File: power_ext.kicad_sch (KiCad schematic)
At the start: 11 parts, among them J1 Conn_01x01, J2 Conn_01x01, J3 Conn_01x01, J4 Conn_01x01, J5 Conn_01x01, J6 Conn_01x01, U132 TLV9061xDBV

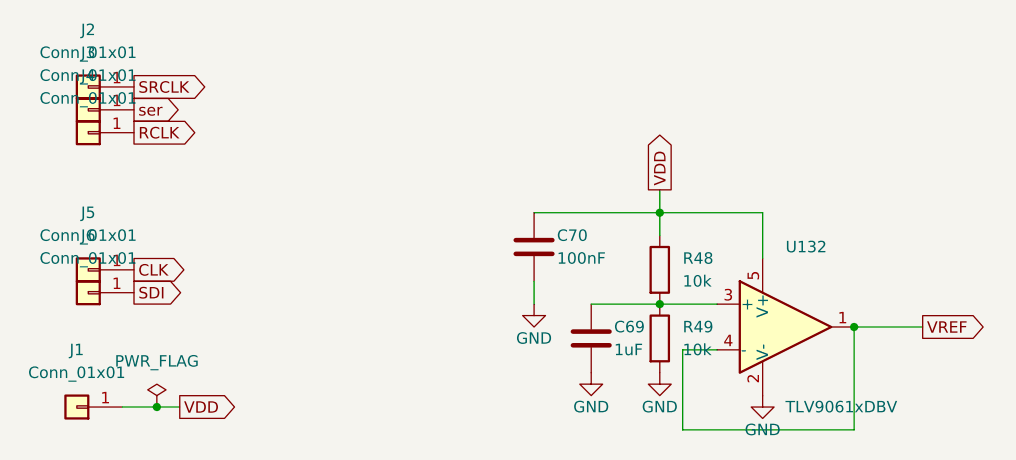
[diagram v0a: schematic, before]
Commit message: Updated: crossbar error
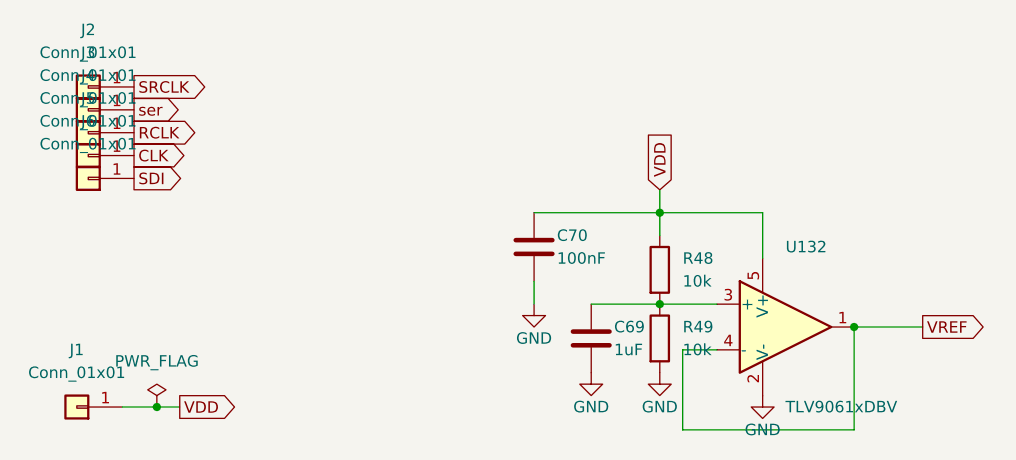
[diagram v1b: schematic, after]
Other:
- moved on the sheet: J5, J6
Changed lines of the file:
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@@
 	)
 	(global_label "VDD"
-		(shape output)
+		(shape input)
 		(at 154.94 88.9 90)
 		(fields_autoplaced yes)
@@
 		)
 		(property "Intersheetrefs" "${INTERSHEET_REFS}"
-			(at 154.94 88.9 0)
-			(effects
-				(font
-					(size 1.27 1.27)
-				)
+			(at 154.94 82.2862 90)
+			(effects
+				(font
+					(size 1.27 1.27)
+				)
+				(justify left)
 				(hide yes)
 			)
@@
 	(global_label "SDI"
 		(shape output)
-		(at 96.52 100.33 0)
+		(at 96.52 87.63 0)
 		(fields_autoplaced yes)
 		(effects
@@
 		)
 		(property "Intersheetrefs" "${INTERSHEET_REFS}"
-			(at 102.5895 100.33 0)
+			(at 102.5895 87.63 0)
 			(effects
 				(font
@@
 	(global_label "CLK"
 		(shape output)
-		(at 96.52 97.79 0)
+		(at 96.52 85.09 0)
 		(fields_autoplaced yes)
 		(effects
@@
 		)
 		(property "Intersheetrefs" "${INTERSHEET_REFS}"
-			(at 103.0733 97.79 0)
+			(at 103.0733 85.09 0)
 			(effects
 				(font
@@
 	(symbol
 		(lib_id "Connector_Generic:Conn_01x01")
-		(at 91.44 100.33 180)
+		(at 91.44 87.63 180)
 		(unit 1)
 		(exclude_from_sim no)
@@
 		(fields_autoplaced yes)
 		(property "Reference" "J6"
-			(at 91.44 93.98 0)
+			(at 91.44 81.28 0)
 			(effects
 				(font
@@
 		)
 		(property "Value" "Conn_01x01"
-			(at 91.44 96.52 0)
+			(at 91.44 83.82 0)
 			(effects
 				(font
@@
 		)
 		(property "Footprint" "analog_NN:WireSolderPad_1.0mm"
-			(at 91.44 100.33 0)
+			(at 91.44 87.63 0)
 			(effects
 				(font
@@
 		)
 		(property "Datasheet" "~"
-			(at 91.44 100.33 0)
+			(at 91.44 87.63 0)
 			(effects
 				(font
@@
 		)
 		(property "Description" "Generic connector, single row, 01x01, script generated (kicad-library-utils/schlib/autogen/connector/)"
-			(at 91.44 100.33 0)
+			(at 91.44 87.63 0)
 			(effects
 				(font
@@
 	(symbol
 		(lib_id "Connector_Generic:Conn_01x01")
-		(at 91.44 97.79 180)
+		(at 91.44 85.09 180)
 		(unit 1)
 		(exclude_from_sim no)
@@
 		(fields_autoplaced yes)
 		(property "Reference" "J5"
-			(at 91.44 91.44 0)
+			(at 91.44 78.74 0)
 			(effects
 				(font
@@
 		)
 		(property "Value" "Conn_01x01"
-			(at 91.44 93.98 0)
+			(at 91.44 81.28 0)
 			(effects
 				(font
@@
 		)
 		(property "Footprint" "analog_NN:WireSolderPad_1.0mm"
-			(at 91.44 97.79 0)
+			(at 91.44 85.09 0)
 			(effects
 				(font
@@
 		)
 		(property "Datasheet" "~"
-			(at 91.44 97.79 0)
+			(at 91.44 85.09 0)
 			(effects
 				(font
@@
 		)
 		(property "Description" "Generic connector, single row, 01x01, script generated (kicad-library-utils/schlib/autogen/connector/)"
-			(at 91.44 97.79 0)
-			(effects
-				(font
+			(at 91.44 85.09 0)
+			(effects
+				(font
